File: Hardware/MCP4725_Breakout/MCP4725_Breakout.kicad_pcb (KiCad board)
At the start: 2 copper layers, 15.2 x 15.2 mm, 17 parts, among them U1 MCP4725

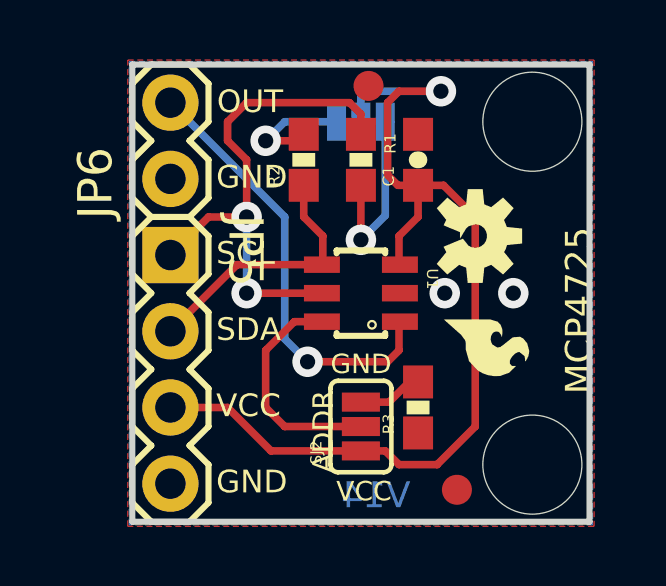
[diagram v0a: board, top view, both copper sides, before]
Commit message: Saves progress
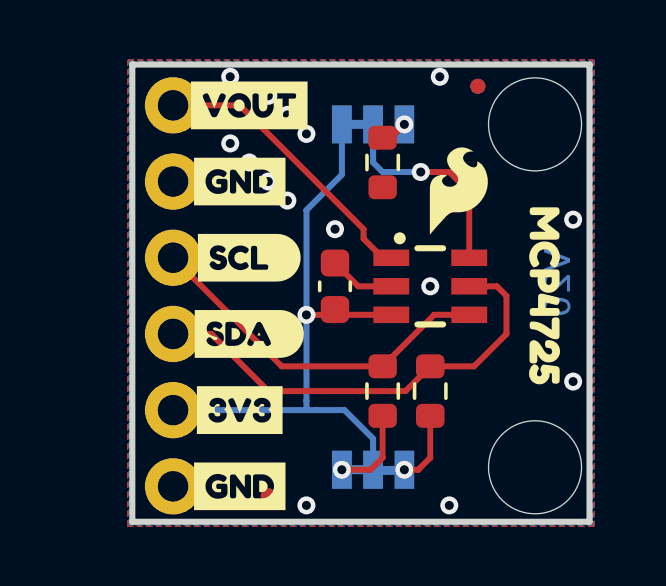
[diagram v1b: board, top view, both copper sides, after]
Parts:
- removed FRAME2: , MCP4725_Breakout:CREATIVE_COMMONS
- removed GND0: LOGO-SFESK, MCP4725_Breakout:SFE-LOGO-FLAME
- removed JP5: , MCP4725_Breakout:1X04
- removed JP6: M02PTH, MCP4725_Breakout:1X02
- removed LOGO1: OSHW-LOGOS, MCP4725_Breakout:OSHW-LOGO-S
- removed R2: 4.7k, MCP4725_Breakout:0603-RES
- removed R3: 10k, MCP4725_Breakout:0603-RES
- removed SJ1: , MCP4725_Breakout:PAD-JUMPER-3-3OF3_NC_BY_TRACE_YES_SILK_FULL_BOX
- removed SJ2: JUMPER-PAD-3-2OF3_NC_BY_PASTE, MCP4725_Breakout:PAD-JUMPER-3-2OF3_NC_BY_PASTE_YES_SILK_FULL_BOX
- removed STANDOFF1, STANDOFF2: STAND-OFF, MCP4725_Breakout:STAND-OFF
- removed U$3: , MCP4725_Breakout:SFE_LOGO_FLAME_.2
- removed U1: MCP4725, MCP4725_Breakout:SOT23-6
- added FID3: Fiducial_0.5mm, SparkFun-Aesthetic:Fiducial_0.5mm_Mask1mm, F.Cu at (145.4, 111.8)
- added FID4: Fiducial_0.5mm, SparkFun-Aesthetic:Fiducial_0.5mm_Mask1mm, B.Cu at (145.4, 111.8)
- added G***: Flame, SparkFun-Aesthetic:SparkFun_Flame_3mm, F.Cu at (151.8, 101.6)
- added G1: OSHW_Logo, SparkFun-Aesthetic:Creative_Commons_License, F.Cu at (175.3, 110.4)
- added J1: Conn_01x02, SparkFun-Connector:1x02_P2.54mm, F.Cu at (142.2, 98.7)
- added J2: I2C, SparkFun-Connector:1x04_P2.54mm, F.Cu at (142.2, 111.4)
- added JP1: I2C, SparkFun-Jumper:Jumper_3_NC-2_Trace, B.Cu at (148.9, 110.9)
- added JP2: ADDR, SparkFun-Jumper:Jumper_3_NC-1_Trace, B.Cu at (148.9, 99.4)
- added R4: 4.7k, SparkFun-Resistor:R_0603_1608Metric, F.Cu at (150.8, 108.3)
- added R5: 4.7k, SparkFun-Resistor:R_0603_1608Metric, F.Cu at (149.2, 108.3)
- added Ref**: Val**, SparkFun-Aesthetic:OSHW_Logo_4mm, B.Cu at (149.5, 105.4)
- added ST1: Standoff, SparkFun-Hardware:Standoff, F.Cu at (154.3, 99.4)
- added ST2: Standoff, SparkFun-Hardware:Standoff, F.Cu at (154.3, 110.8)
- added U2: MCP4725, SparkFun-Semiconductor-Standard:SOT23-6, F.Cu at (150.8, 104.8)
- added kibuzzard-69B46D81: G***, kibuzzard-69B46D81, F.Cu at (144.8, 98.7)
- added kibuzzard-69B46D81: G***, kibuzzard-69B46D81, B.Cu at (144.8, 98.7)
- added kibuzzard-69B46D94: G***, kibuzzard-69B46D94, F.Cu at (144.5, 111.4)
- added kibuzzard-69B46D94: G***, kibuzzard-69B46D94, F.Cu at (144.5, 101.3)
- added kibuzzard-69B46D94: G***, kibuzzard-69B46D94, B.Cu at (144.5, 101.3)
- added kibuzzard-69B46D94: G***, kibuzzard-69B46D94, B.Cu at (144.5, 111.4)
- added kibuzzard-69B46DE0: G***, kibuzzard-69B46DE0, F.Cu at (144.5, 108.9)
- added kibuzzard-69B46DE0: G***, kibuzzard-69B46DE0, B.Cu at (144.5, 108.9)
- added kibuzzard-69B46E1A: G***, kibuzzard-69B46E1A, F.Cu at (154.6, 105.1)
- added kibuzzard-69B46E1A: G***, kibuzzard-69B46E1A, B.Cu at (153.0, 105.1)
- added kibuzzard-69B46E2A: G***, kibuzzard-69B46E2A, F.Cu at (144.8, 103.8)
- added kibuzzard-69B46E2F: G***, kibuzzard-69B46E2F, F.Cu at (144.8, 106.4)
- added kibuzzard-69B46E79: G***, kibuzzard-69B46E79, B.Cu at (148.9, 101.3)
- added kibuzzard-69B46E88: G***, kibuzzard-69B46E88, B.Cu at (148.9, 108.9)
- added kibuzzard-69B46EE5: G***, kibuzzard-69B46EE5, B.Cu at (144.8, 106.4)
- added kibuzzard-69B46EEC: G***, kibuzzard-69B46EEC, B.Cu at (144.8, 103.8)
- C1: footprint MCP4725_Breakout:0603-CAP -> SparkFun-Capacitor:C_0603_1608Metric
- FID1: value FIDUCIAL1X2 -> Fiducial_0.5mm; footprint MCP4725_Breakout:FIDUCIAL-1X2 -> SparkFun-Aesthetic:Fiducial_0.5mm_Mask1mm; moved to B.Cu
- FID2: value FIDUCIAL1X2 -> Fiducial_0.5mm; footprint MCP4725_Breakout:FIDUCIAL-1X2 -> SparkFun-Aesthetic:Fiducial_0.5mm_Mask1mm
- R1: value 4.7k -> 10k; footprint MCP4725_Breakout:0603-RES -> SparkFun-Resistor:R_0603_1608Metric
- moved FID1 13.5 mm to (152.4, 98.1), turned to 180 degrees
- moved C1 5.04 mm to (147.6, 104.8)
- moved FID2 3.64 mm to (152.4, 98.1)
- moved R1 0.73 mm to (149.2, 100.6), turned to 90 degrees
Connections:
- C1 pad 1: VCC -> 3.3V
- R1 pad 1: SCL -> GND
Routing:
- net VCC: track 32.8 -> 0.00 mm, vias 1 -> 0
- net 3.3V: track 0.00 -> 21.1 mm, vias 0 -> 1
- net N$3: track 7.61 -> 0.00 mm
- net ADDR: track 0.00 -> 7.08 mm, vias 0 -> 1
- net SDA: track 8.89 -> 15.3 mm
- net Net-(JP2-C): track 6.09 -> 0.91 mm
- net VOUT: track 14.7 -> 9.56 mm, vias 1 -> 0
- net SCL: track 17.1 -> 12.1 mm, vias 2 -> 0
- net N$1: track 3.98 -> 0.00 mm, vias 1 -> 0
- net Net-(JP1-A): track 0.00 -> 2.92 mm, vias 0 -> 1
- net Net-(JP1-C): track 0.00 -> 2.43 mm, vias 0 -> 1
- net GND: track 0.00 -> 2.20 mm, vias 2 -> 16
- net N$4: track 2.18 -> 0.00 mm
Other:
- rule pad_to_mask_clearance: 0 -> 0.127
- board text added: "V20"
- board text removed: "ADDR"
- board text removed: "GND"
- board text removed: "I2C"
- board text removed: "Joel Bartlett"
- board text removed: "MCP4725"
- board text removed: "OUT"
- board text removed: "PULLUPS"
- board text removed: "SCL"
- board text removed: "SDA"
- board text removed: "V14"
- board text removed: "VCC"
